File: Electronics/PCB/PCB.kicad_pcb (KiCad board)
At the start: 2 copper layers, 100 x 70 mm, 19 parts, among them J2 CONN_NIDEC_0, J3 CONN_NIDEC_1, J4 CONN_ESP32_L, J5 CONN_ESP32_R, J6 CONN_MPU6050, J7 Conn_Coaxial_Power, U3 LM7805_TO220

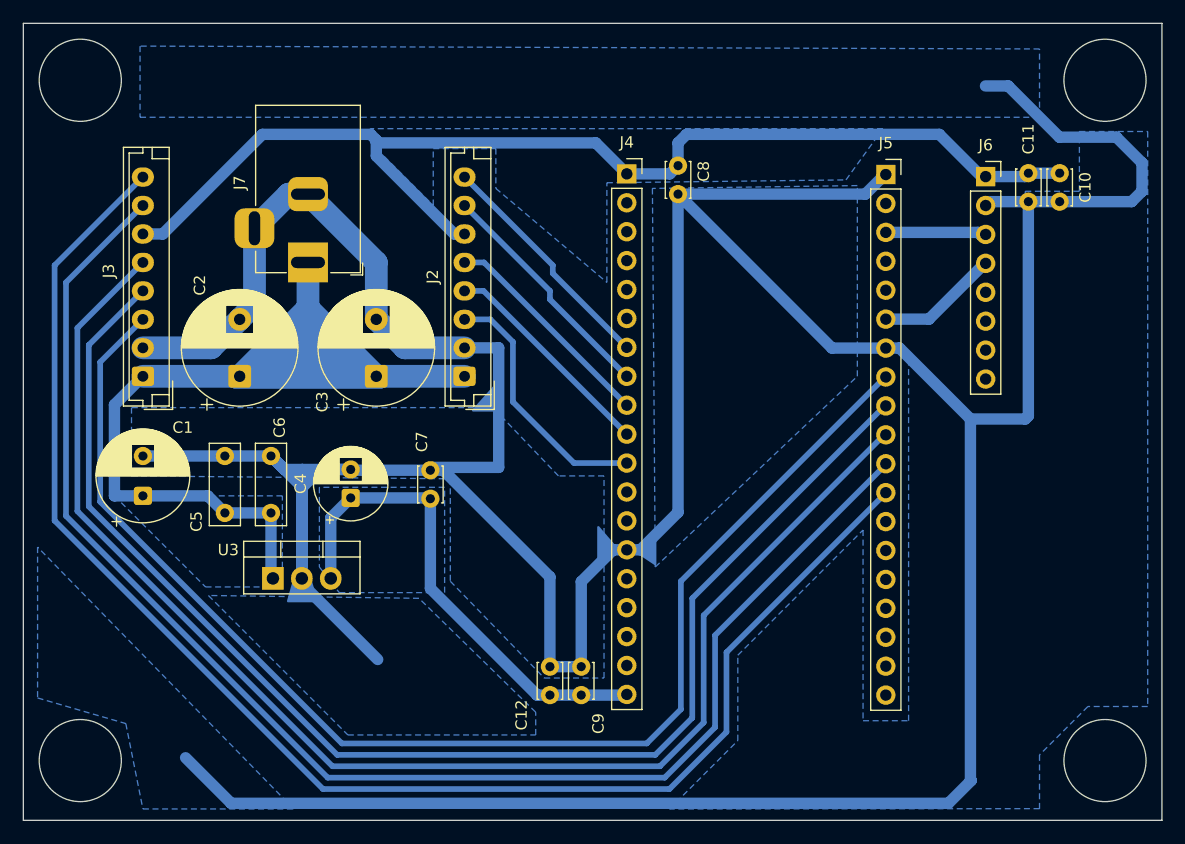
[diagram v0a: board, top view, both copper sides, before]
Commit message: fix pcb
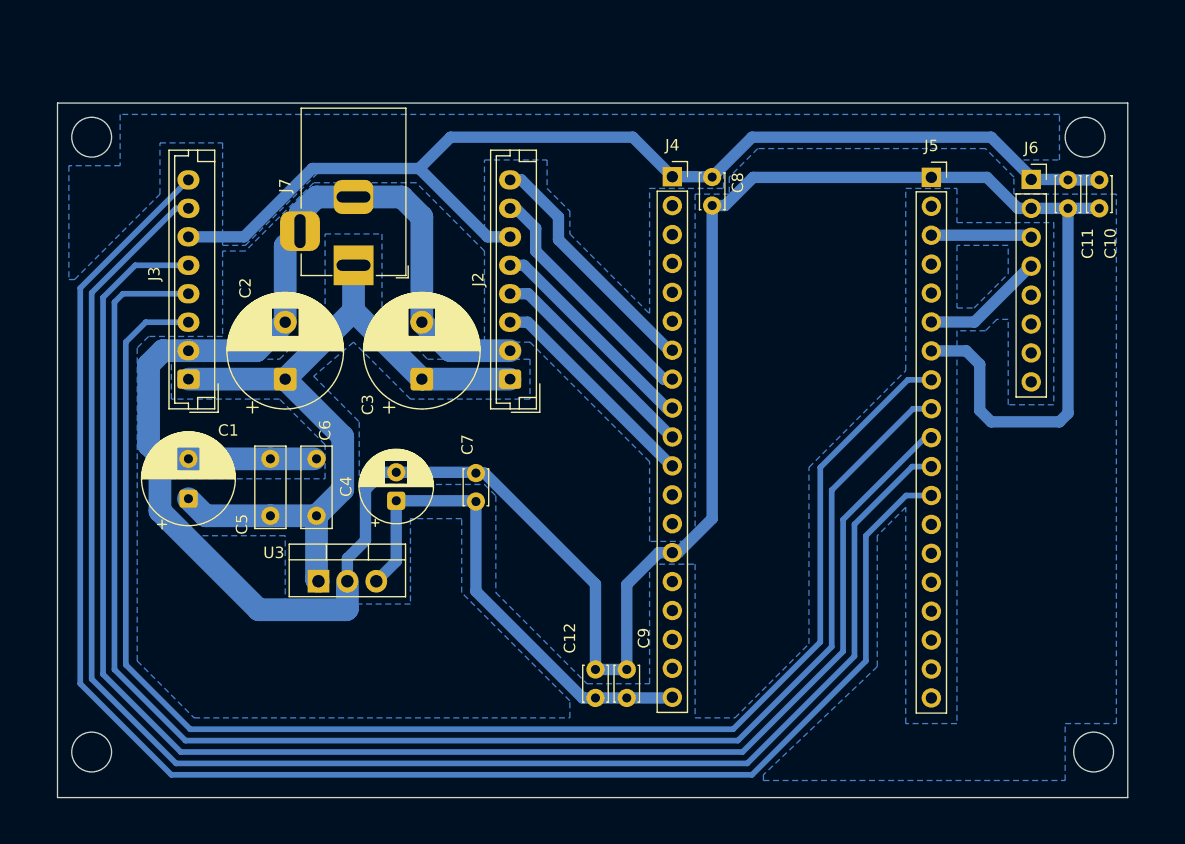
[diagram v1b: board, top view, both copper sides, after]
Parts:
- moved C1 4.01 mm to (144.5, 90.8)
- moved C12 4.01 mm to (180.2, 108.2)
- moved C2 4.01 mm to (153.0, 80.2)
- moved C3 4.01 mm to (165.0, 80.2)
- moved C4 4.01 mm to (162.8, 90.9)
- moved C5 4.01 mm to (151.7, 92.2)
- moved C6 4.01 mm to (155.8, 92.2)
- moved C7 4.01 mm to (169.8, 91.0)
- moved C9 4.01 mm to (183.0, 108.2)
- moved J2 4.01 mm to (172.8, 80.2)
- moved J3 4.01 mm to (144.5, 80.2)
- moved J4 4.01 mm to (187.0, 62.5)
- moved J5 4.01 mm to (209.8, 62.5)
- moved J6 4.01 mm to (218.5, 62.7)
- moved J7 4.01 mm to (159.0, 70.2)
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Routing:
- net GND: track 421.1 -> 264.7 mm
- net /M1_PWM: track 118.8 -> 133.5 mm
- net /M1_BRK: track 115.3 -> 129.3 mm
- net /M1_DIR: track 122.1 -> 135.6 mm
- net /M1_ENC_A: track 127.8 -> 139.9 mm
- net /M1_ENC_B: track 131.1 -> 142.9 mm
- net /M0_BRK: track 22.6 -> 19.5 mm
- net +3.3V: track 101.5 -> 98.7 mm
- net +12V: track 68.9 -> 70.0 mm
- net /M0_ENC_B: track 20.9 -> 21.6 mm
- net /M0_ENC_A: track 20.9 -> 21.6 mm
- added copper zone on B.Cu, net (none)
- removed copper zone on B.Cu, net +12V
- removed copper zone on B.Cu, net +5V
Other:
- board size 100 x 70 mm -> 94 x 61 mm
